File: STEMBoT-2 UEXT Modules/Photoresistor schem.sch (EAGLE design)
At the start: 3 parts

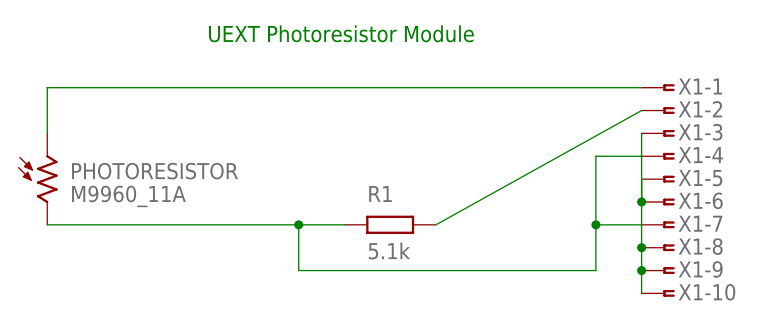
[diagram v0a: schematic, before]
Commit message: Update Photoresistor schem.sch
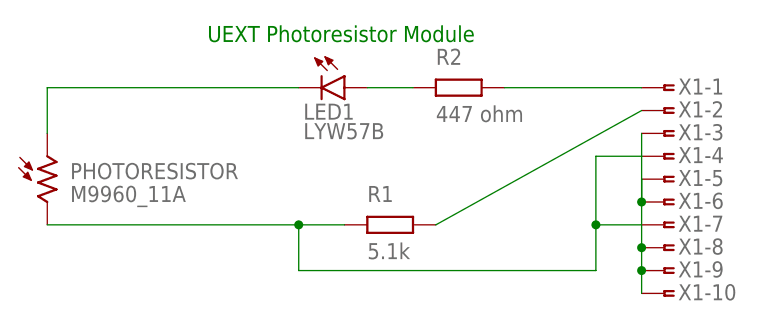
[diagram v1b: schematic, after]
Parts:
- added LED1: LYW57B, led:LYW57B
- added R2: 447 ohm, ngspice-simulation:R
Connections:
- new net N$4: R2.2, X1-1.1
- new net N$6: LED1.A, R2.1
- net N$3: now also LED1.C; no longer X1-1.1
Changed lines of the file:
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@@
 <part name="X1" library="con-amp" library_urn="urn:adsk.eagle:library:127" deviceset="FSIDE-10" device="" package3d_urn="urn:adsk.eagle:package:8081495/1"/>
 <part name="R1" library="ngspice-simulation" library_urn="urn:adsk.eagle:library:527439" deviceset="R" device="" value="5.1k"/>
+<part name="R2" library="ngspice-simulation" library_urn="urn:adsk.eagle:library:527439" deviceset="R" device="" value="447 ohm"/>
+<part name="LED1" library="led" library_urn="urn:adsk.eagle:library:259" deviceset="*W57B" device="" package3d_urn="urn:adsk.eagle:package:15859/1" technology="LY"/>
 </parts>
 <sheets>
@@
 <attribute name="VALUE" x="93.98" y="62.23" size="1.778" layer="96"/>
 </instance>
+<instance part="R2" gate="G$1" x="104.14" y="81.28" smashed="yes">
+<attribute name="NAME" x="101.6" y="83.82" size="1.778" layer="95"/>
+<attribute name="VALUE" x="101.6" y="77.47" size="1.778" layer="96"/>
+</instance>
+<instance part="LED1" gate="G$1" x="91.44" y="81.28" smashed="yes" rot="R270">
+<attribute name="NAME" x="86.868" y="77.724" size="1.778" layer="95"/>
+<attribute name="VALUE" x="86.868" y="75.565" size="1.778" layer="96"/>
+</instance>
 </instances>
 <busses>
@@
 <net name="N$3" class="0">
 <segment>
-<pinref part="X1" gate="-1" pin="1"/>
-<wire x1="124.46" y1="81.28" x2="58.42" y2="81.28" width="0.1524" layer="91"/>
 <pinref part="PHOTORESISTOR" gate="G$1" pin="1"/>
 <wire x1="58.42" y1="76.2" x2="58.42" y2="81.28" width="0.1524" layer="91"/>
+<wire x1="86.36" y1="81.28" x2="58.42" y2="81.28" width="0.1524" layer="91"/>
+<pinref part="LED1" gate="G$1" pin="C"/>
 </segment>
 </net>
@@
 </segment>
 </net>
+<net name="N$4" class="0">
+<segment>
+<pinref part="X1" gate="-1" pin="1"/>
+<wire x1="124.46" y1="81.28" x2="109.22" y2="81.28" width="0.1524" layer="91"/>
+<pinref part="R2" gate="G$1" pin="2"/>
+</segment>
+</net>
+<net name="N$6" class="0">
+<segment>
+<pinref part="R2" gate="G$1" pin="1"/>
+<wire x1="99.06" y1="81.28" x2="93.98" y2="81.28" width="0.1524" layer="91"/>
+<pinref part="LED1" gate="G$1" pin="A"/>
+</segment>
+</net>
